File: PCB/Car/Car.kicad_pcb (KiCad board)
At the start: 2 copper layers, 70 x 100 mm, 10 parts, among them J1 L1, J2 L2, J3 R1, J4 R2, J5 Conn_01x02_Pin, J6 Conn_01x02_Pin, J7 Conn_01x03, J8 Conn_01x06, U2 YAAJ_DCDC_StepDown_LM2596, U3 YAAJ_DCDC_StepDown_LM2596

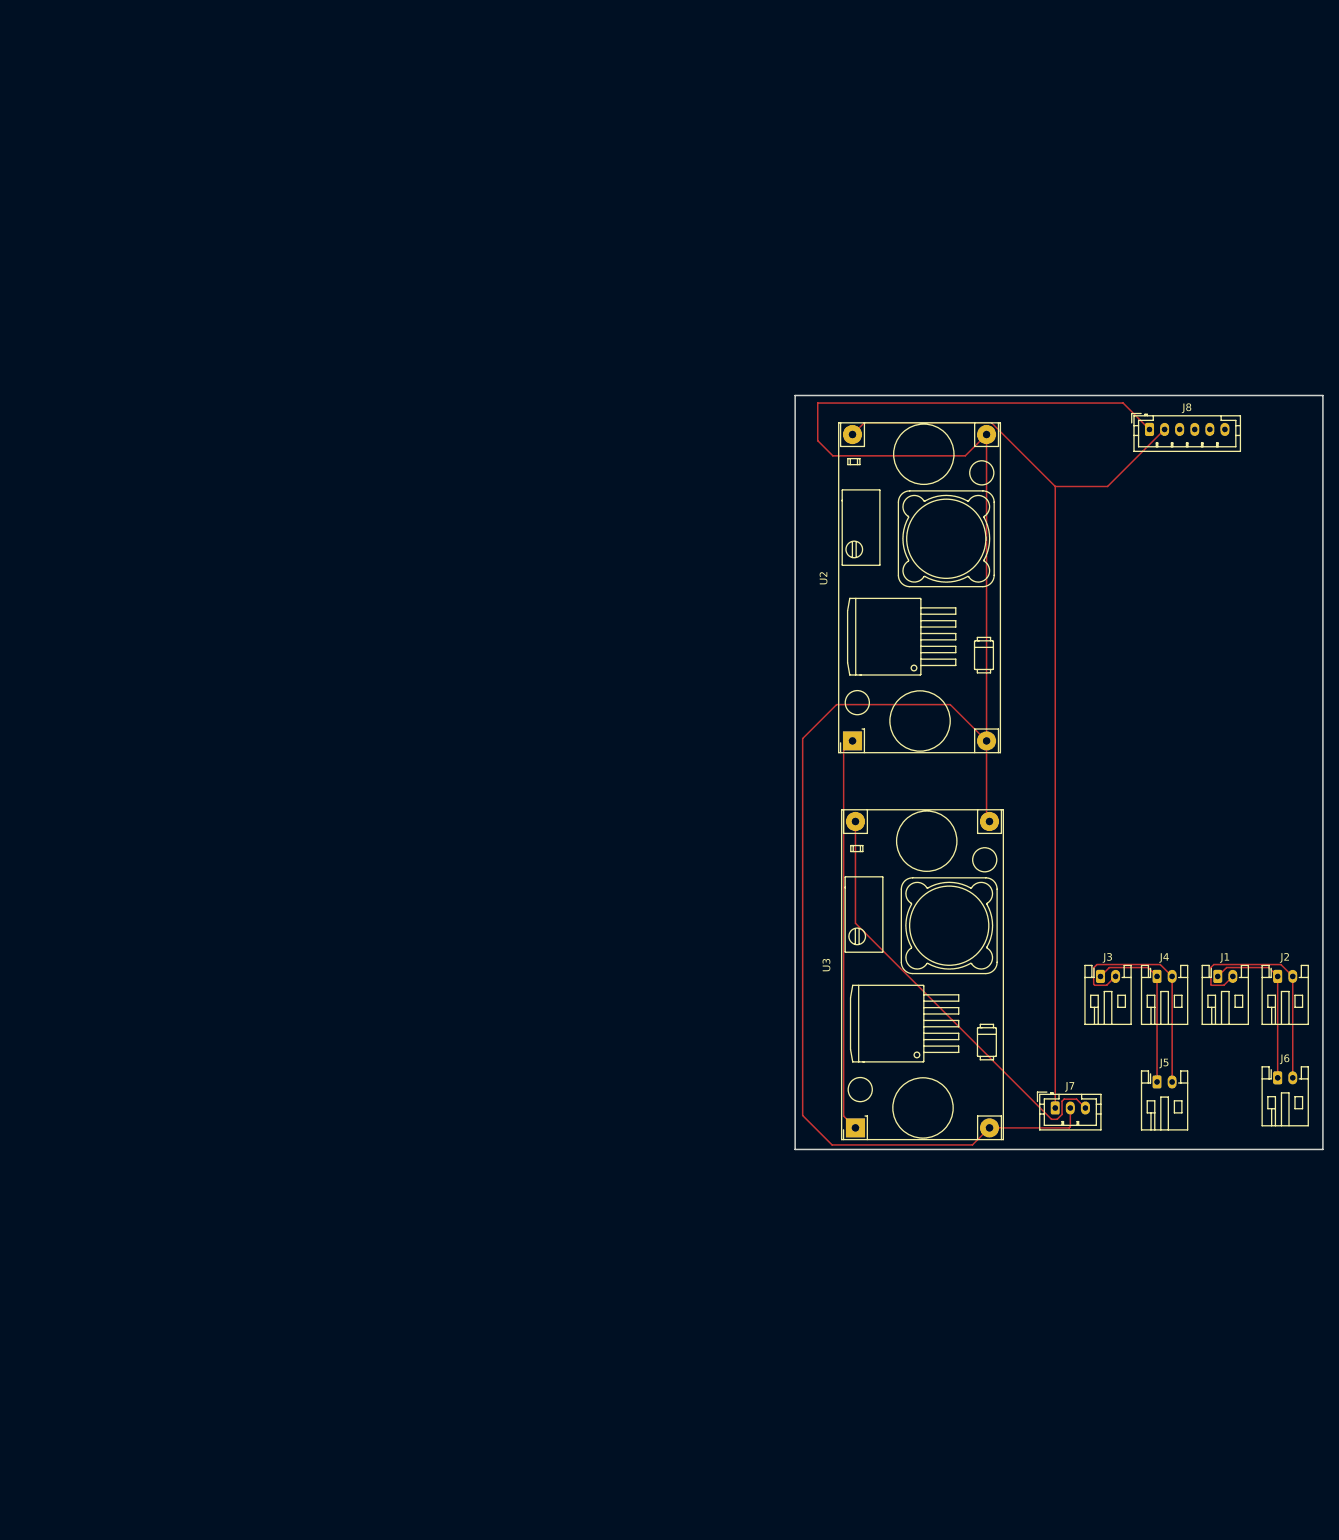
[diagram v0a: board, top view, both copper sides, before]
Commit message: finish PCB
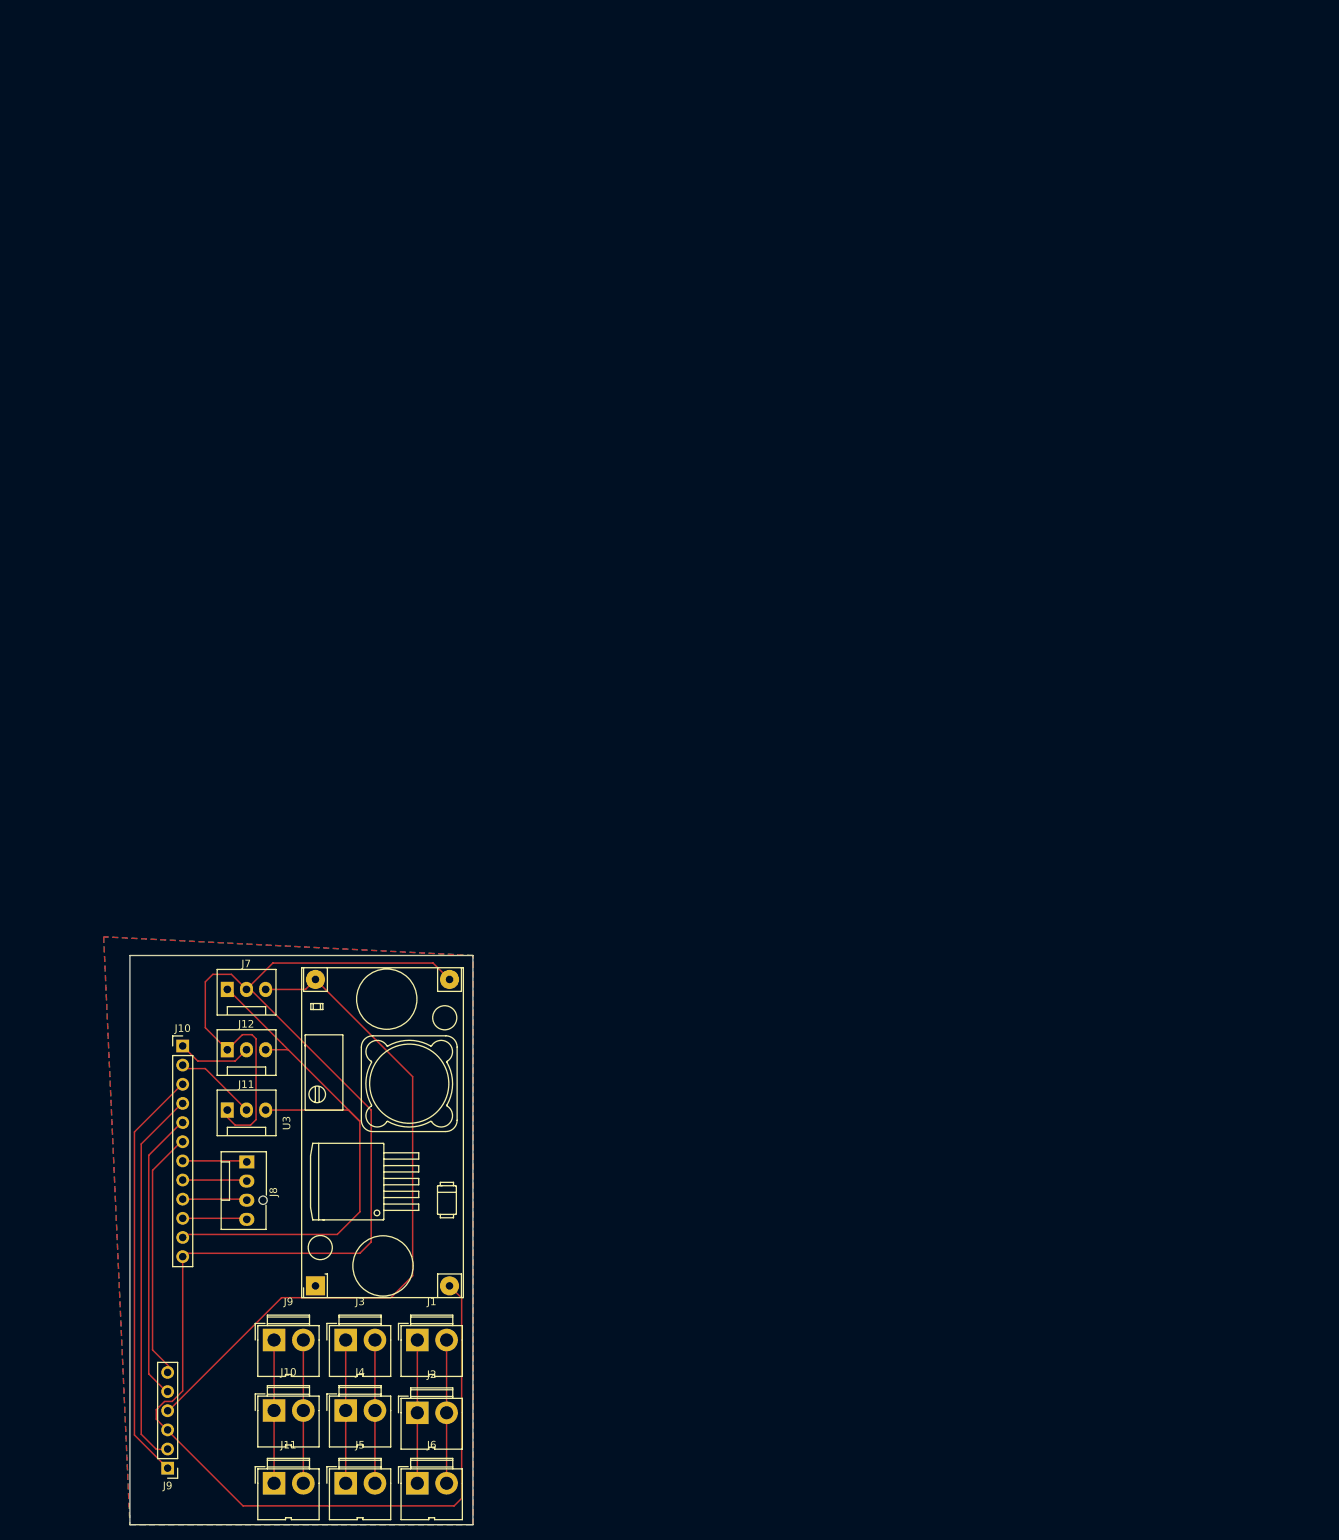
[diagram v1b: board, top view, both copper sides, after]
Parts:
- removed U2: YAAJ_DCDC_StepDown_LM2596, lm2596:YAAJ_DCDC_StepDown_LM2596
- added J10: FL2, Connector:JWT_A3963_1x02_P3.96mm_Vertical, F.Cu at (30.9, 182.6)
- added J10: Conn_01x12, Connector_PinHeader_2.54mm:PinHeader_1x12_P2.54mm_Vertical, F.Cu at (18.8, 134.3)
- added J11: Conn_01x03, Connector:FanPinHeader_1x03_P2.54mm_Vertical, F.Cu at (24.7, 142.8)
- added J11: FLT, Connector:JWT_A3963_1x02_P3.96mm_Vertical, F.Cu at (30.9, 192.3)
- added J12: Conn_01x03, Connector:FanPinHeader_1x03_P2.54mm_Vertical, F.Cu at (24.7, 134.8)
- added J9: Conn_01x06, Connector_PinHeader_2.54mm:PinHeader_1x06_P2.54mm_Vertical, F.Cu at (16.8, 190.3)
- added J9: FL1, Connector:JWT_A3963_1x02_P3.96mm_Vertical, F.Cu at (30.9, 173.3)
- J1, J2, J3, J4: footprint Connector_JST:JST_PH_S2B-PH-K_1x02_P2.00mm_Horizontal -> Connector:JWT_A3963_1x02_P3.96mm_Vertical
- J5: value Conn_01x02_Pin -> R1+2; footprint Connector_JST:JST_PH_S2B-PH-K_1x02_P2.00mm_Horizontal -> Connector:JWT_A3963_1x02_P3.96mm_Vertical
- J6: value Conn_01x02_Pin -> L1+2; footprint Connector_JST:JST_PH_S2B-PH-K_1x02_P2.00mm_Horizontal -> Connector:JWT_A3963_1x02_P3.96mm_Vertical
- J7: footprint Connector_JST:JST_PH_B3B-PH-K_1x03_P2.00mm_Vertical -> Connector:FanPinHeader_1x03_P2.54mm_Vertical
- J8: value Conn_01x06 -> Conn_01x04; footprint Connector_JST:JST_PH_B6B-PH-K_1x06_P2.00mm_Vertical -> Connector:FanPinHeader_1x04_P2.54mm_Vertical
- moved J8 154.2 mm to (27.3, 149.7), turned to -90 degrees
- moved J2 127.9 mm to (49.9, 182.9)
- moved J6 126.1 mm to (49.9, 192.3)
- moved J4 122.0 mm to (40.4, 182.6)
- moved J5 120.1 mm to (40.4, 192.3)
- moved J1 116.6 mm to (49.9, 173.3)
- moved J3 111.1 mm to (40.4, 173.3)
- moved J7 110.9 mm to (24.7, 126.8)
- moved U3 74.6 mm to (36.4, 166.1)
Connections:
- net +6V renamed +6.5V
- J8 pad 1: GND -> IN4
- J8 pad 2: +5V -> IN3
- J8 pad 3: IN4 -> IN2
- J8 pad 4: IN3 -> IN1
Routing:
- net BA: track 0.00 -> 55.5 mm
- net +5V: track 131.1 -> 77.7 mm
- net VCC: track 52.5 -> 0.00 mm
- net BB: track 0.00 -> 50.6 mm
- net AA: track 0.00 -> 38.9 mm
- net +6.5V: track 57.4 -> 91.8 mm
- net AB: track 0.00 -> 34.0 mm
- net Net-(J10-Pin_2): track 0.00 -> 19.3 mm
- net Net-(J10-Pin_1): track 0.00 -> 19.3 mm
- net GND: track 245.2 -> 232.4 mm
- net Net-(J3-Pin_2): track 30.9 -> 19.0 mm
- net Net-(J1-Pin_2): track 30.8 -> 19.0 mm
- net LED1: track 0.00 -> 11.0 mm
- net LED2: track 0.00 -> 9.91 mm
- net IN2: track 0.00 -> 8.56 mm
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- added copper zone on B.Cu, net GND
- added copper zone on F.Cu, net GND
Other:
- board size 70 x 100 mm -> 45.5 x 75.5 mm

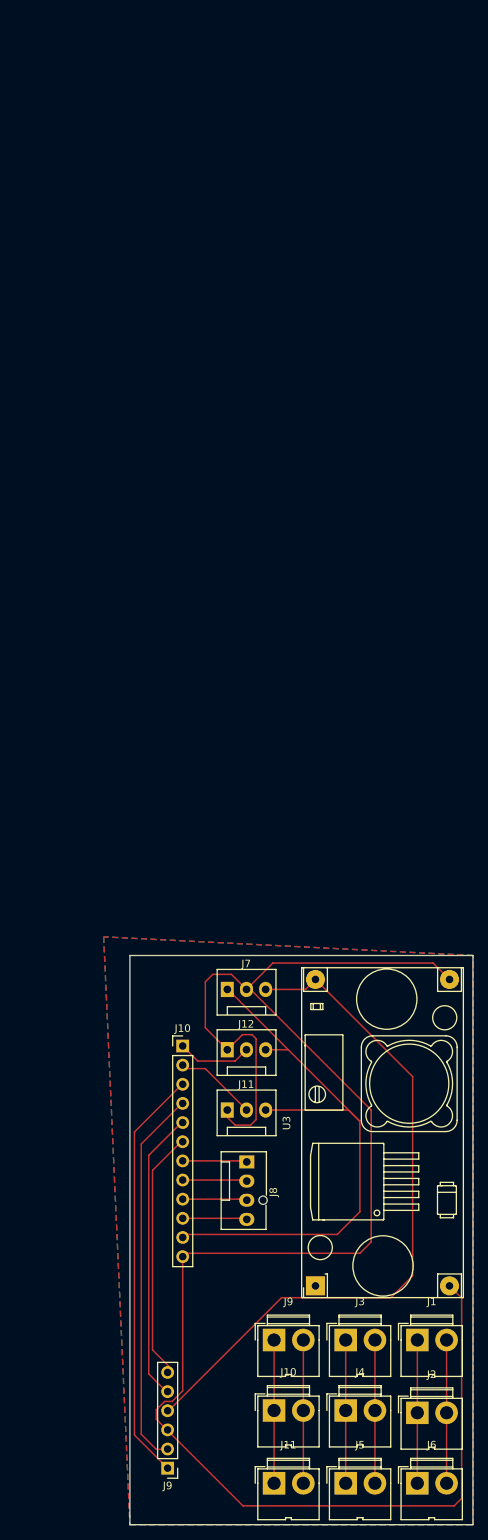
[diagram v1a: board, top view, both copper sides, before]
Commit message: updated firmware
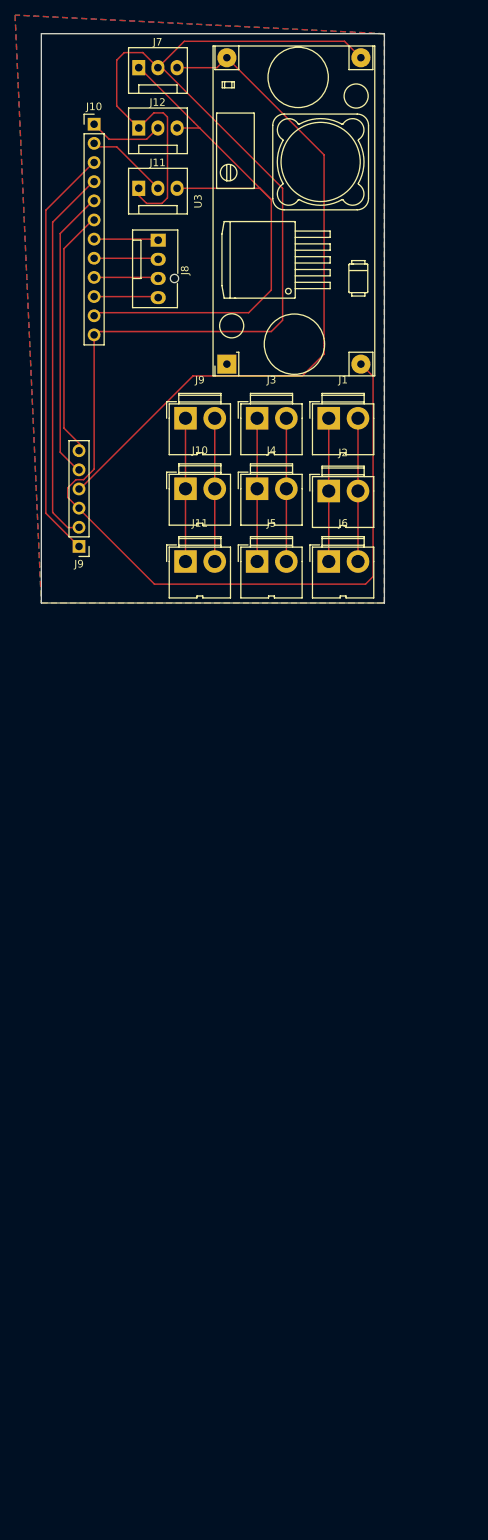
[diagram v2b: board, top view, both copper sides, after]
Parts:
- moved J10 122.8 mm to (7.02, 12.0)
- moved J11 122.8 mm to (12.9, 20.5)
- moved J11 122.8 mm to (19.1, 70.0)
- moved J12 122.8 mm to (12.9, 12.5)
- moved J2 122.8 mm to (38.1, 60.7)
- moved J5 122.8 mm to (28.6, 70.0)
- moved J6 122.8 mm to (38.1, 70.0)
- moved J7 122.8 mm to (12.9, 4.52)
- moved J9 122.8 mm to (5.02, 68.0)
- moved J1 122.8 mm to (38.1, 51.0)
- moved J10 122.8 mm to (19.1, 60.4)
- moved J3 122.8 mm to (28.6, 51.0)
- moved J4 122.8 mm to (28.6, 60.4)
- moved J8 122.8 mm to (15.5, 27.4)
- moved J9 122.8 mm to (19.1, 51.0)
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
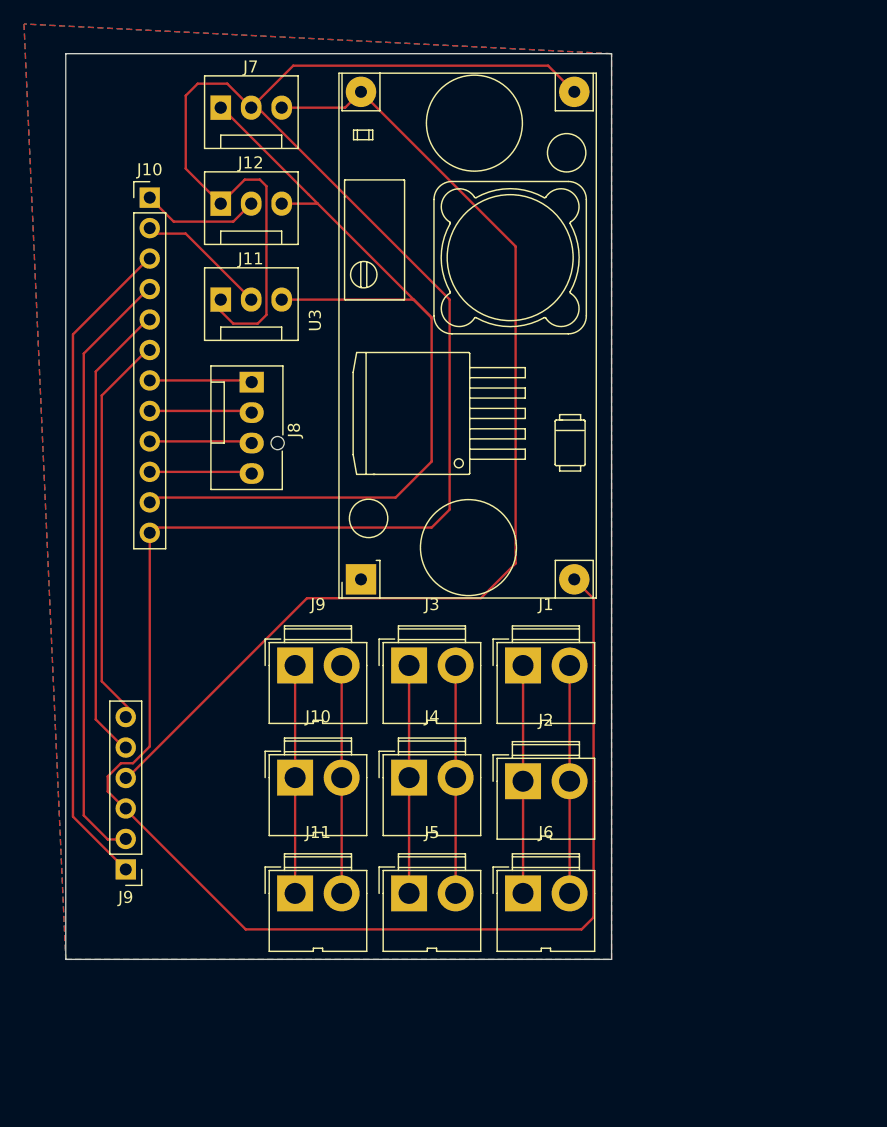
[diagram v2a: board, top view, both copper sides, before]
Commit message: updated pcb :D
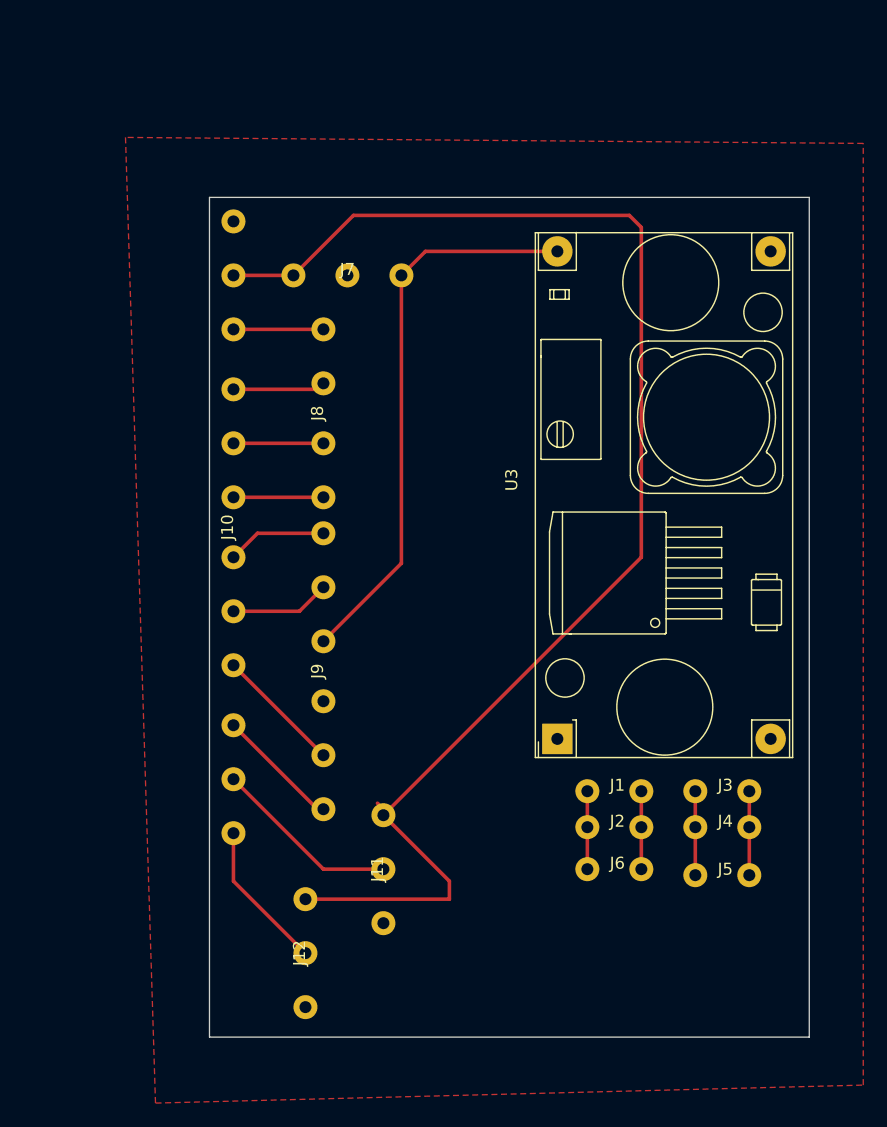
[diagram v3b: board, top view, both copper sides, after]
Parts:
- removed the J10 at (19.1, 60.4)
- removed the J10 at (7.02, 12.0)
- removed the J11 at (12.9, 20.5)
- removed the J11 at (19.1, 70.0)
- removed the J9 at (5.02, 68.0)
- removed the J9 at (19.1, 51.0)
- added J10: Conn_01x12, JST:JST 1x12, F.Cu at (14.0, 39.5)
- added J11: Conn_01x03, JST:JST 1x3, F.Cu at (26.5, 68.0)
- added J9: Conn_01x06, JST:JST 1x6, F.Cu at (21.5, 51.5)
- J1, J2, J3, J4, J5, J6: footprint Connector:JWT_A3963_1x02_P3.96mm_Vertical -> JST:JST 1x2
- J12, J7: footprint Connector:FanPinHeader_1x03_P2.54mm_Vertical -> JST:JST 1x3
- J8: footprint Connector:FanPinHeader_1x04_P2.54mm_Vertical -> JST:JST 1x4
- moved J12 62.9 mm to (20.0, 75.0), turned to 90 degrees
- moved J3 28.4 mm to (55.0, 61.5)
- moved J4 26.7 mm to (55.0, 64.5)
- moved J5 26.4 mm to (55.0, 68.5)
- moved U3 21.1 mm to (41.0, 57.1)
- moved J7 17.5 mm to (23.5, 18.5)
- moved J1 13.1 mm to (46.0, 61.5)
- moved J2 8.74 mm to (46.0, 64.5)
- moved J6 8.12 mm to (46.0, 68.0)
- moved J8 6.52 mm to (21.5, 30.0), turned to 90 degrees
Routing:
- net GND: track 232.4 -> 0.00 mm
- net BA: track 55.5 -> 10.4 mm
- net +6.5V: track 91.8 -> 47.0 mm
- net BB: track 50.6 -> 10.6 mm
- net +5V: track 77.7 -> 116.9 mm
- net AA: track 38.9 -> 8.33 mm
- net AB: track 34.0 -> 8.33 mm
- net Net-(J10-Pin_2): track 19.3 -> 0.00 mm
- net Net-(J10-Pin_1): track 19.3 -> 0.00 mm
- net Net-(J1-Pin_2): track 19.0 -> 6.50 mm
- net Net-(J1-Pin_1): track 19.0 -> 6.50 mm
- net Net-(J3-Pin_2): track 19.0 -> 7.00 mm
- net Net-(J3-Pin_1): track 19.0 -> 7.00 mm
- net LED1: track 11.0 -> 15.6 mm
- net LED2: track 9.91 -> 12.5 mm
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- removed copper zone on B.Cu, net GND
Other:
- board size 45.5 x 75.5 mm -> 50 x 70 mm
